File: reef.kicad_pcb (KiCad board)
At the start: 2 copper layers, 87 parts, among them J1 nice!view sockets, J2 battery connector, SW0 B3U-1000P[], SW1 PCM12SMTR, U1 nice_nano, U2 TRRS, U3 TRRS

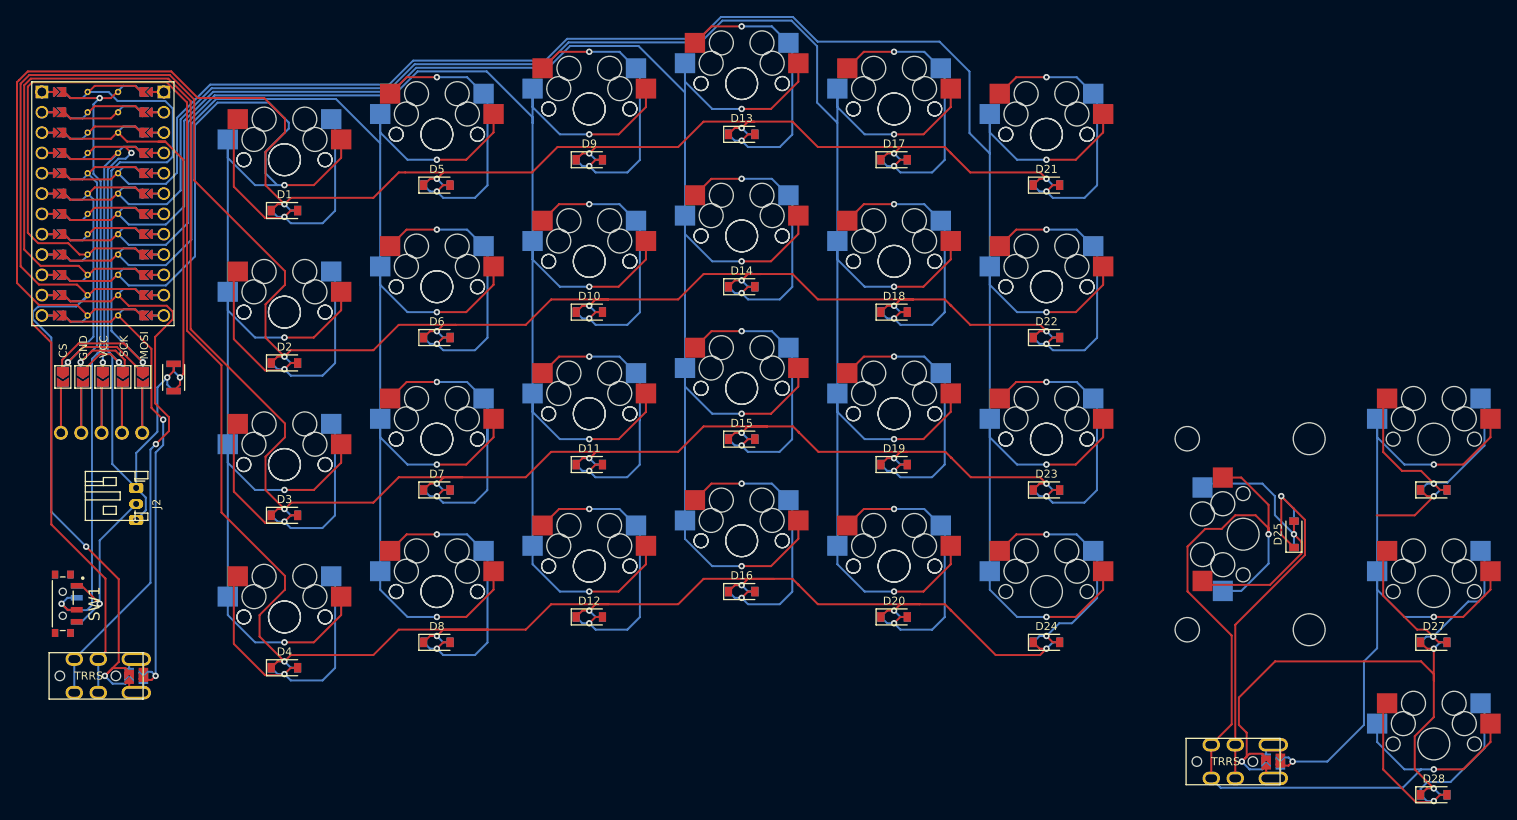
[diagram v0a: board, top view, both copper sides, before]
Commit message: Teardrops and Fillets
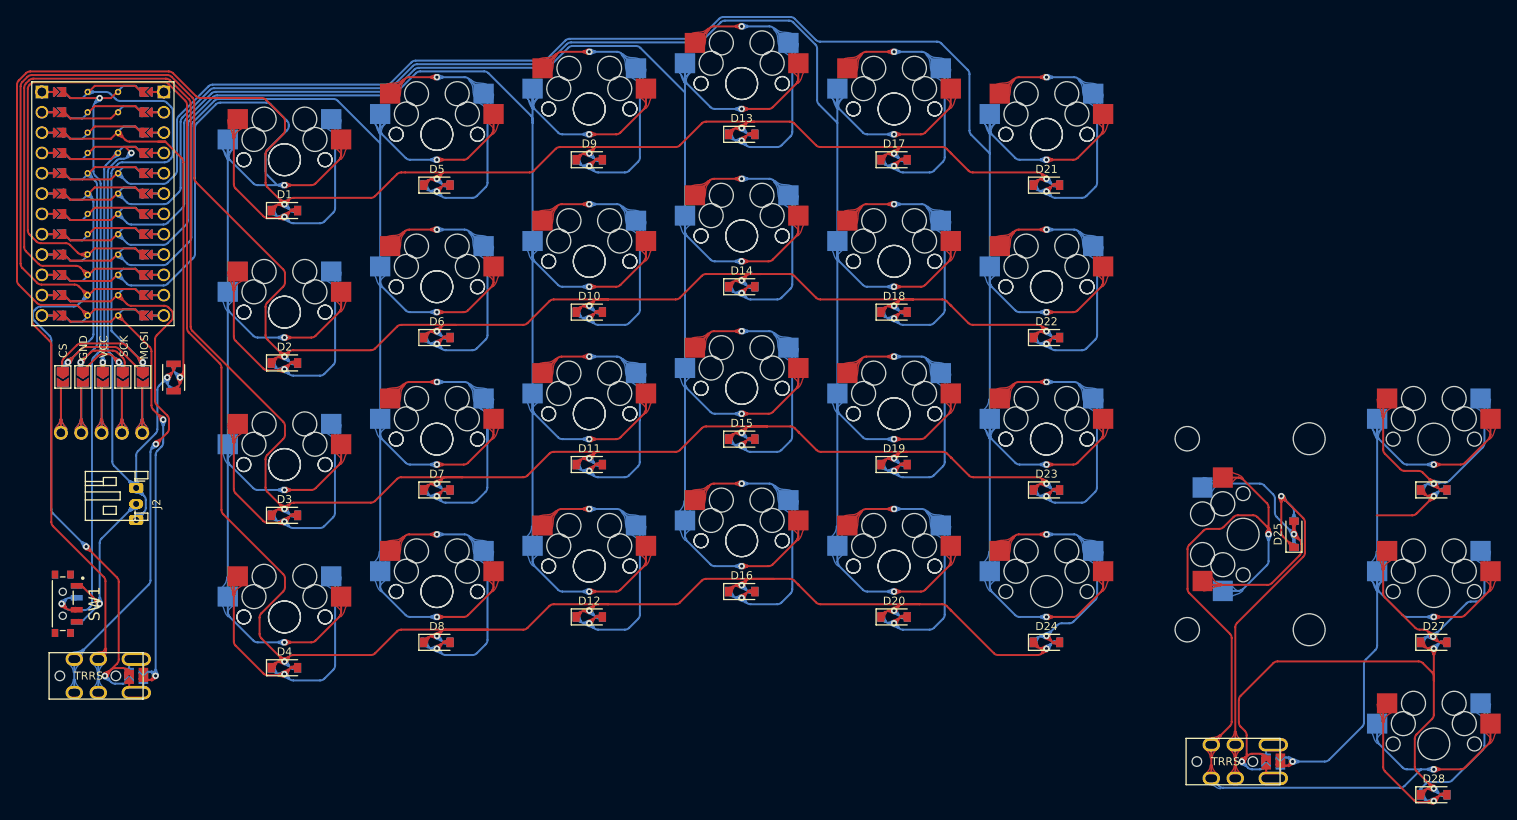
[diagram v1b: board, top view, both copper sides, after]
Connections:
- Display1 pad 1: (no net) -> disp_1
- Display1 pad 2: (no net) -> disp_2
- Display1 pad 3: (no net) -> disp_3
- Display1 pad 4: (no net) -> disp_4
- Display1 pad 5: (no net) -> disp_5
- J1 pad 10: (no net) -> disp_1
- J1 pad 6: (no net) -> disp_1
- J1 pad 7: (no net) -> disp_2
- J1 pad 8: (no net) -> disp_3
- J1 pad 9: (no net) -> disp_4
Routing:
- net (no net): track 63.3 -> 0.00 mm
- net disp_1: track 0.00 -> 12.7 mm
- net disp_2: track 0.00 -> 12.7 mm
- net disp_3: track 0.00 -> 12.7 mm
- net disp_4: track 0.00 -> 12.6 mm
- net disp_5: track 0.00 -> 12.6 mm
- net row_1: track 297.8 -> 295.9 mm
- net row_3: track 270.7 -> 269.1 mm
- net row_0: track 270.0 -> 268.4 mm
- net row_2: track 248.3 -> 246.8 mm
- net col_5: track 277.3 -> 276.1 mm
- net col_4: track 258.2 -> 257.1 mm
- net col_0: track 195.2 -> 194.2 mm
- net col_3: track 232.9 -> 231.9 mm
- net col_2: track 215.3 -> 214.4 mm
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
